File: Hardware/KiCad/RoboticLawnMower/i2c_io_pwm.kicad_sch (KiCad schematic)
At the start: 6 parts, among them U4 PCA9685PW, U5 PCA9557PW

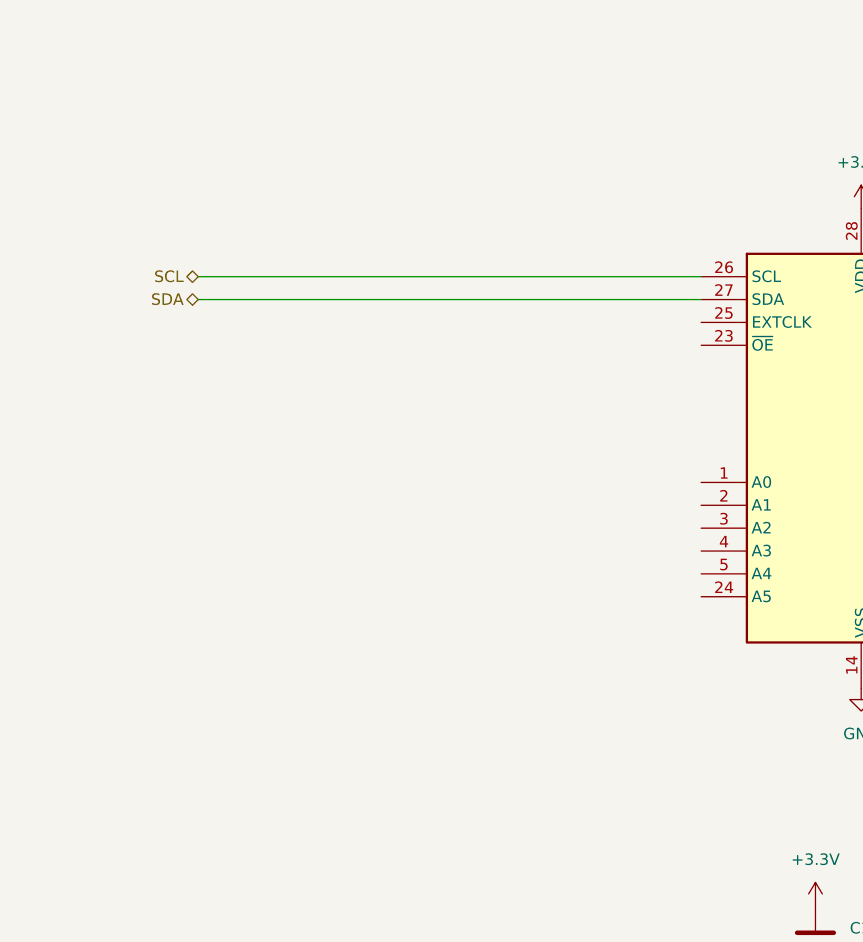
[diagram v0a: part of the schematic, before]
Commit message: schaltplan und layout
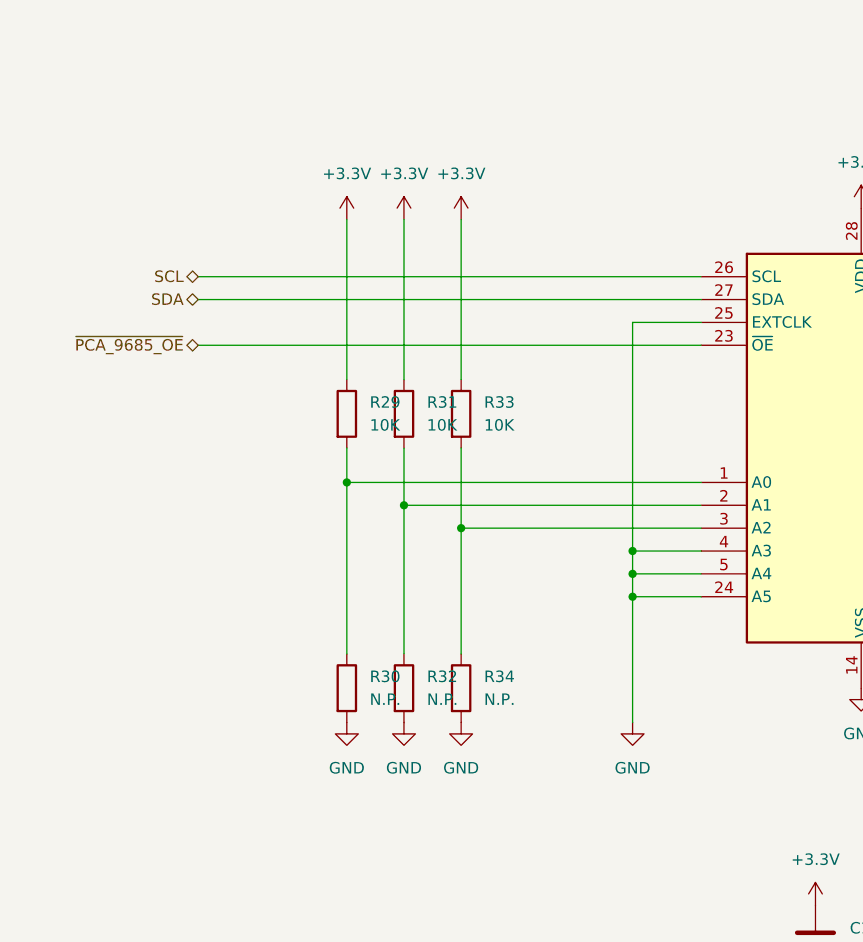
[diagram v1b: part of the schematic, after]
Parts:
- added R29, R31, R33: 10K, Resistor_SMD:R_0402_1005Metric, symbol Device:R
- added R30, R32, R34: N.P., Resistor_SMD:R_0402_1005Metric, symbol Device:R
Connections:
- net +3.3V: now also R29.1, R31.1, R33.1
- net GND: now also U4.24 (A5), U4.25 (EXTCLK), U4.4 (A3), U4.5 (A4), R30.2, R32.2, R34.2
- net at U4.1 (A0): now also R29.2, R30.1
- net at U4.2 (A1): now also R31.2, R32.1
- net ~{PCA_9685_OE}: now reaches U4.23 (~{OE})
- net at U4.3 (A2): now also R33.2, R34.1
